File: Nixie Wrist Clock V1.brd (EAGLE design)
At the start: 88.1 x 64.2 mm, 39 parts, among them Q1 310mA/60V/1.6Ω, Q2 310mA/60V/1.6Ω, Q3 310mA/60V/1.6Ω, Q4 310mA/60V/1.6Ω, Q5 310mA/60V/1.6Ω, U2 NRF52832, X3 32MHz, X4 32.768kHz

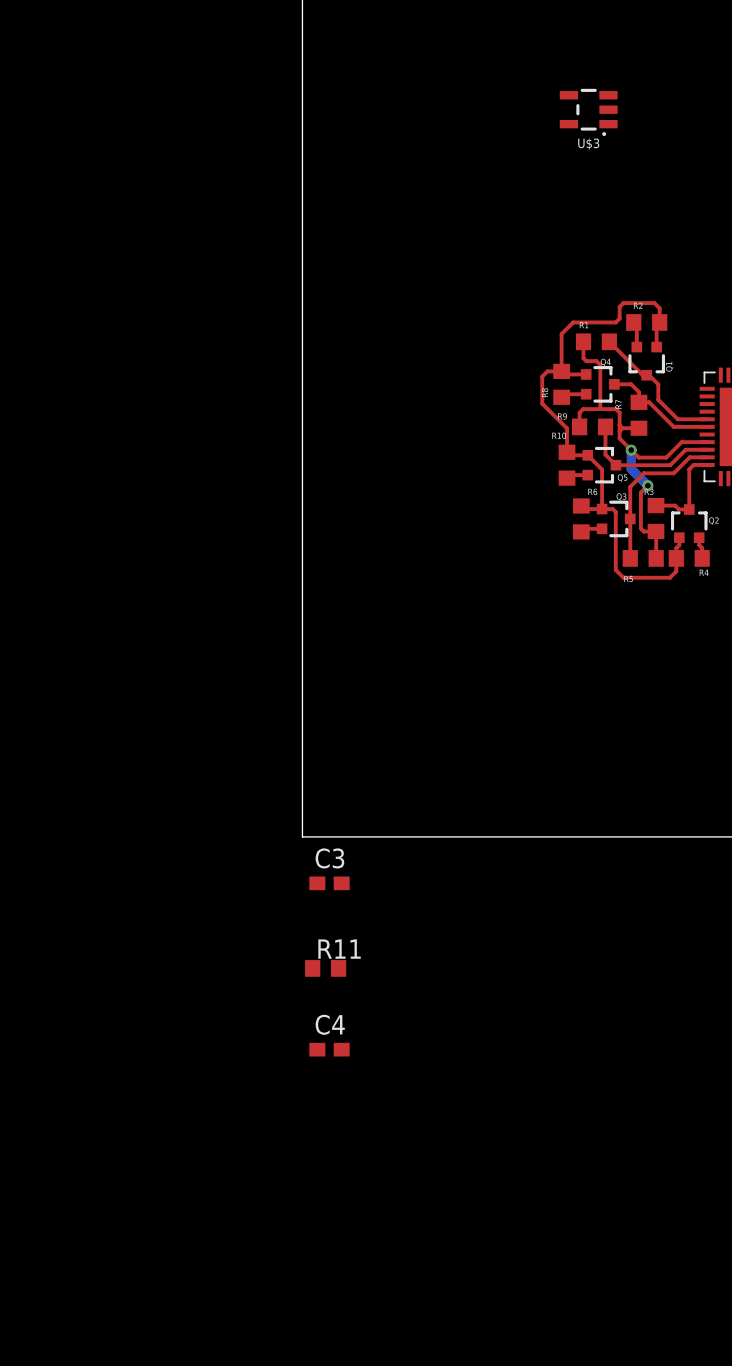
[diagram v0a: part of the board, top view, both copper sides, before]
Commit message: Update #6
5V Supply IC added
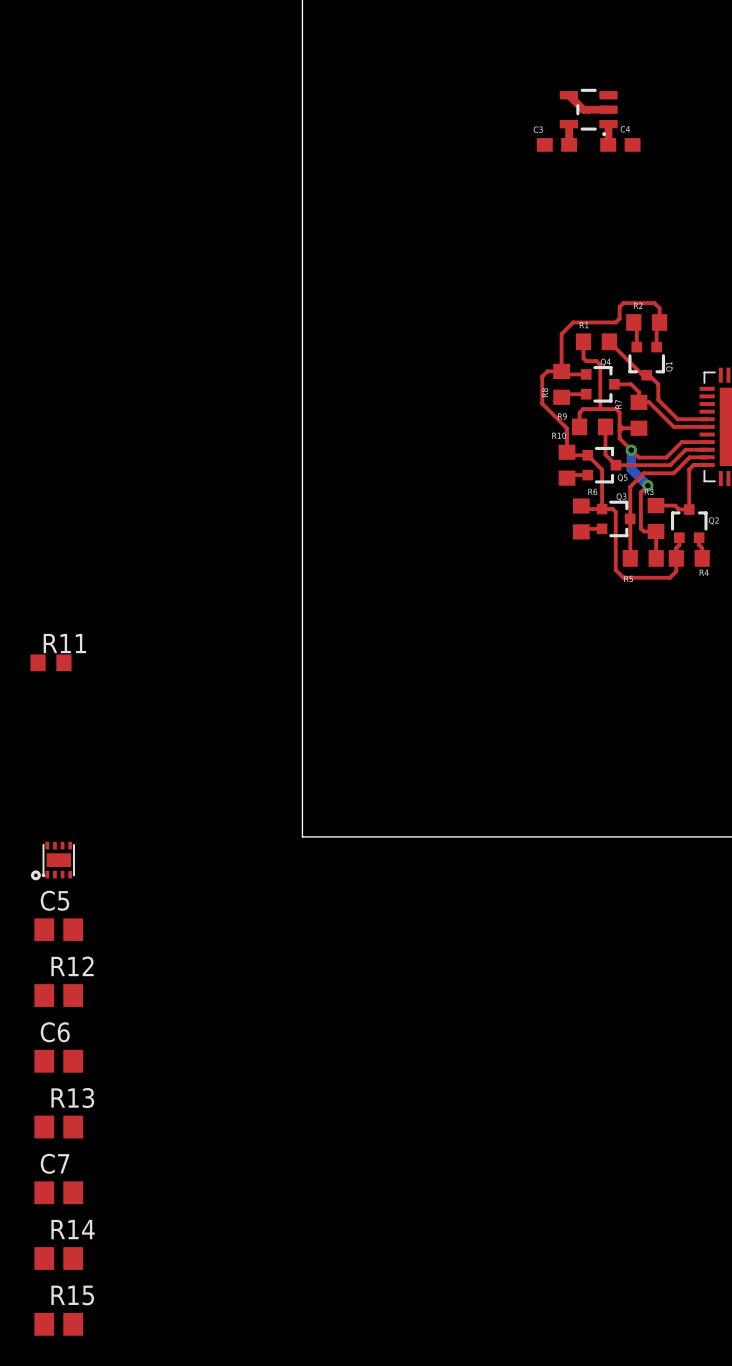
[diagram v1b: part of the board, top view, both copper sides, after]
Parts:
- added C5: 10uF, rcl:C0805
- added C6: 100pF, rcl:C0805
- added C7: 22uF, rcl:C0805
- added R12: 316K, rcl:R0805
- added R13: 100K, rcl:R0805
- added R14: 868K, rcl:R0805
- added R15: 6.65K, rcl:R0805
- added U$4: TPS61252DSGR, Alp-Special:WSON-8-PAD
- moved C4 62.4 mm to (20.9, 45.4)
- moved C3 50.7 mm to (16.7, 45.4), turned to 180 degrees
- moved R11 27.0 mm to (-16.5, 11.4)
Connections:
- new net 5V-SUPPLY-ENA: U$4.6
- new net N$10: R14.1, U$4.5
- new net N$12: C5.1, U$4.8
- new net N$13: U$4.7
- new net N$15: C6.2, R12.1, R13.2, U$4.3
- new net N$2: R15.2, U$4.4
- net +5V: now also C6.1, C7.1, R12.2, R14.2, U$4.2
- net GND: now also C5.2, C7.2, R13.1, R15.1, U$4.1, U$4.PAD
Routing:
- net GND: track 25.3 -> 28.3 mm
- net +3V3: track 72.0 -> 73.4 mm
- net VCC: track 0.00 -> 1.37 mm

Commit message: Revert "Update #6"
This reverts commit 39989620e637334a808b500ab2563335b83f3b38.
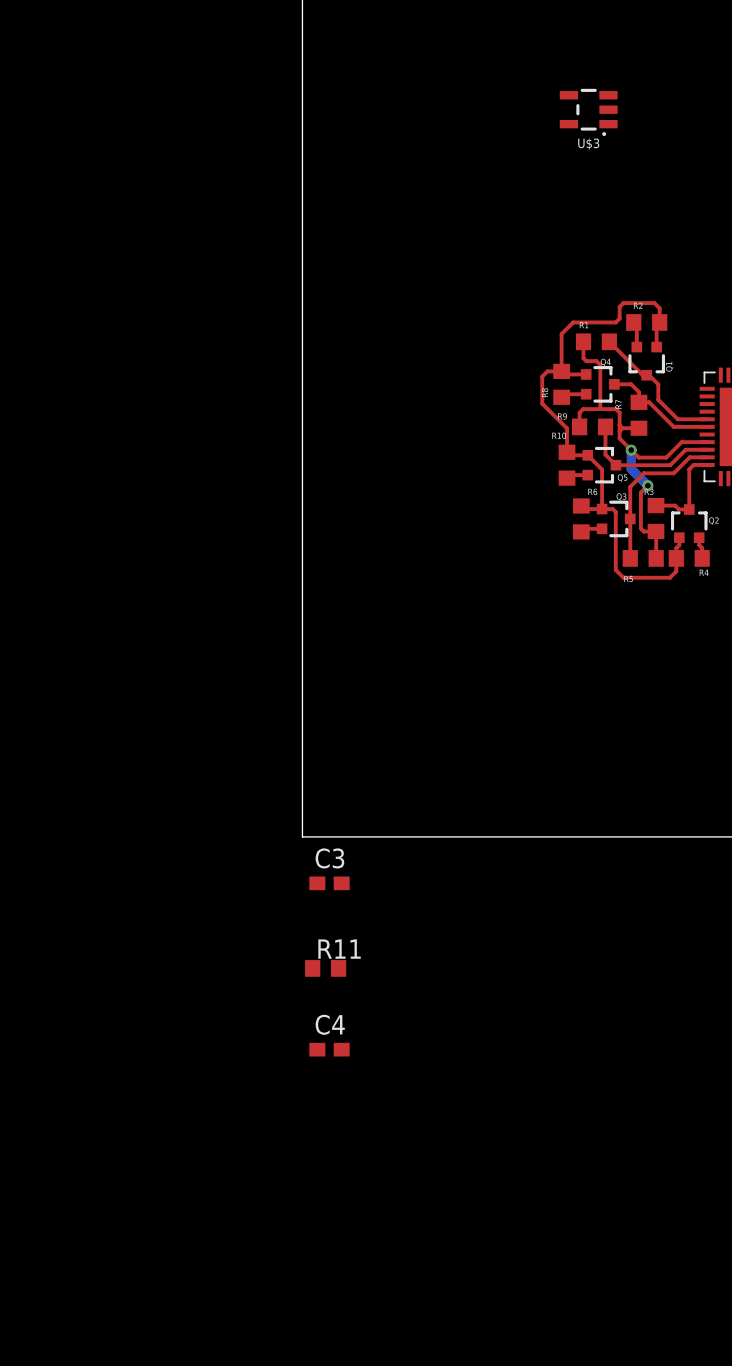
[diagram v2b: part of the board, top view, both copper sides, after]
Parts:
- removed C5: 10uF, rcl:C0805
- removed C6: 100pF, rcl:C0805
- removed C7: 22uF, rcl:C0805
- removed R12: 316K, rcl:R0805
- removed R13: 100K, rcl:R0805
- removed R14: 868K, rcl:R0805
- removed R15: 6.65K, rcl:R0805
- removed U$4: TPS61252DSGR, Alp-Special:WSON-8-PAD
- moved C4 62.4 mm to (1.78, -14.0)
- moved C3 50.7 mm to (1.78, -3.05), turned to 0 degrees
- moved R11 27.0 mm to (1.52, -8.64)
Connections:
- removed net 5V-SUPPLY-ENA: U$4.6
- removed net N$10: R14.1, U$4.5
- removed net N$12: C5.1, U$4.8
- removed net N$13: U$4.7
- removed net N$15: C6.2, R12.1, R13.2, U$4.3
- removed net N$2: R15.2, U$4.4
- net +5V: no longer C6.1, C7.1, R12.2, R14.2, U$4.2
- net GND: no longer C5.2, C7.2, R13.1, R15.1, U$4.1, U$4.PAD
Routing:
- net GND: track 28.3 -> 25.3 mm
- net +3V3: track 73.4 -> 72.0 mm
- net VCC: track 1.37 -> 0.00 mm
